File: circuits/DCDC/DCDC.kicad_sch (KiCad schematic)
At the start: 2 parts, among them Q7 2N7002

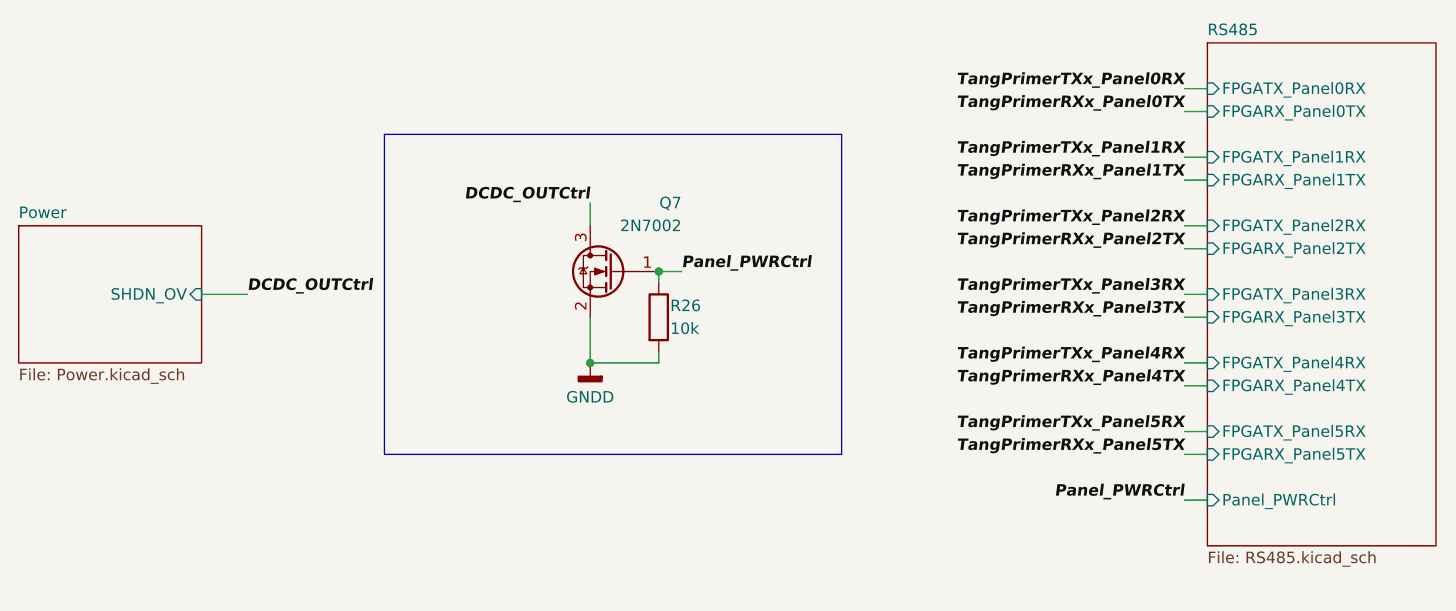
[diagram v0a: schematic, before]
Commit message: 発注第3弾
DCDC、MD追加
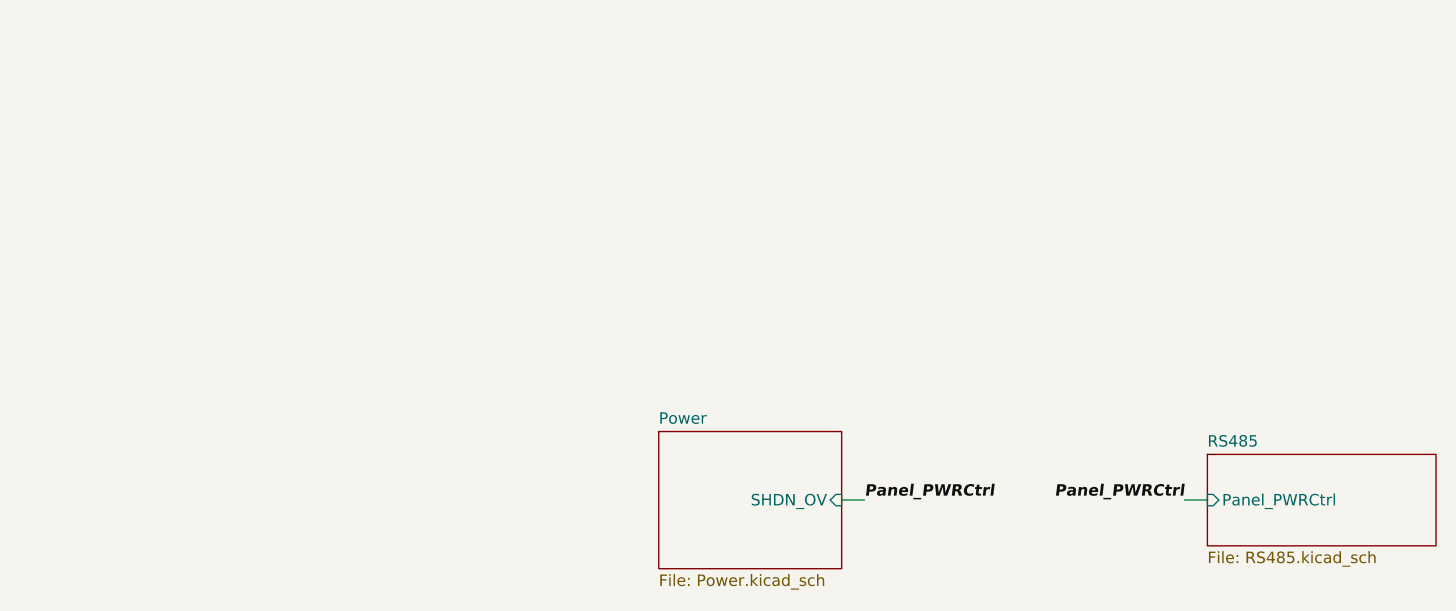
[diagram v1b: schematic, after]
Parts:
- removed Q7: 2N7002, Package_TO_SOT_SMD:SOT-23, symbol Transistor_FET:2N7002
- removed R26: 10k, Resistor_SMD:R_0402_1005Metric, symbol Device:R
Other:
- sheet RS485 ports: added none; removed FPGARX_Panel0TX, FPGARX_Panel1TX, FPGARX_Panel2TX, FPGARX_Panel3TX, FPGARX_Panel4TX, FPGARX_Panel5TX, FPGATX_Panel0RX, FPGATX_Panel1RX, FPGATX_Panel2RX, FPGATX_Panel3RX, FPGATX_Panel4RX, FPGATX_Panel5RX
